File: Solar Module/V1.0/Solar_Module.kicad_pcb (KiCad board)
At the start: 4 copper layers, 23 parts, among them J1 B2B-PH-K-S, J2 TYPE-C16PIN, J3 B2B-PH-K-S, U1 MT3608, U2 TP4057

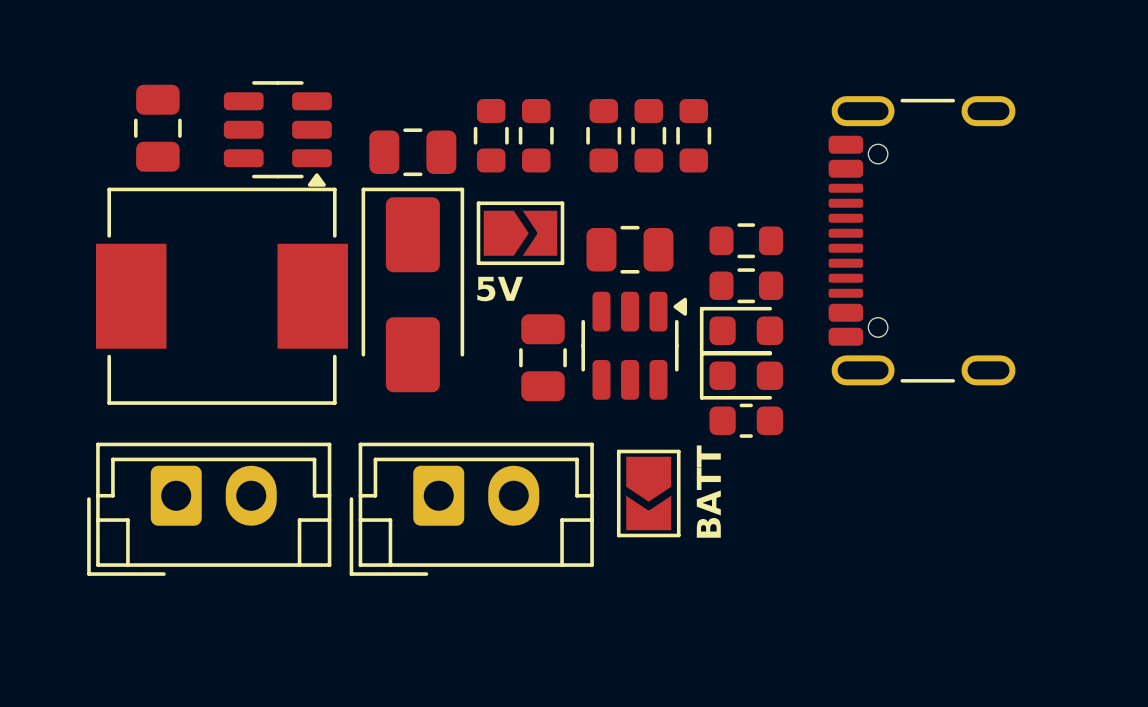
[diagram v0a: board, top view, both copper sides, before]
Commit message: Design roughly finished. Now Routing.
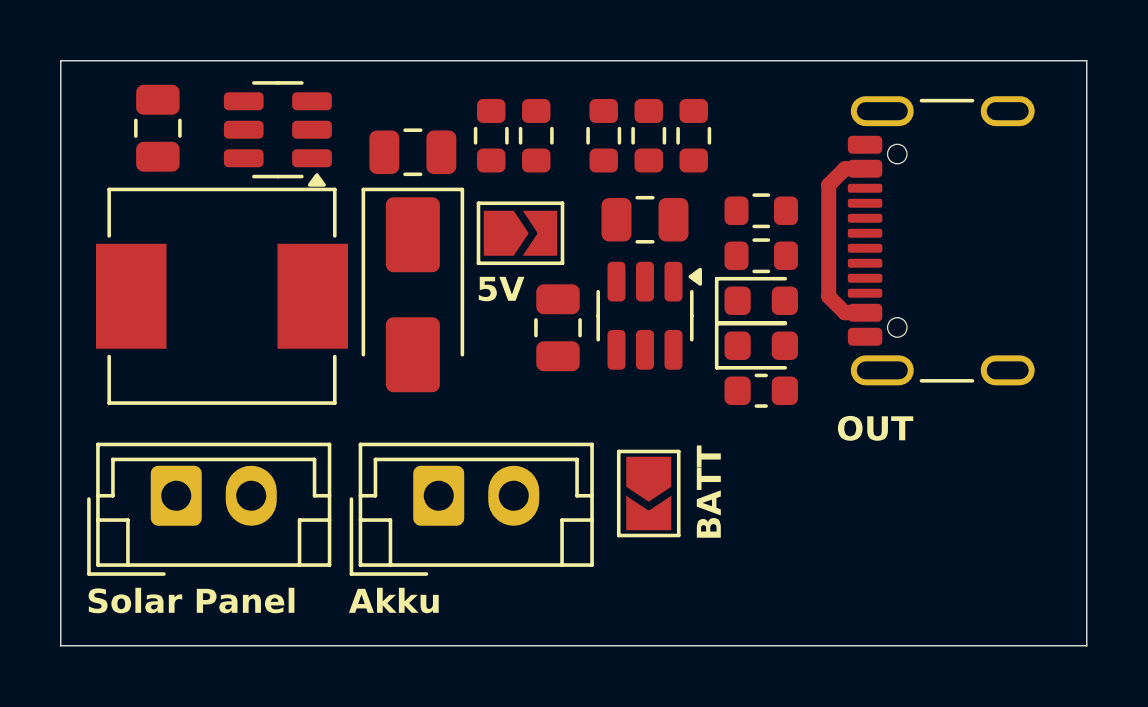
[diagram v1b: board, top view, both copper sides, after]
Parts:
- moved C3 1.12 mm to (168.0, 65.4)
- moved C4 1.12 mm to (170.9, 61.8)
- moved D2 1.12 mm to (174.8, 64.5)
- moved D3 1.12 mm to (174.8, 66.0)
- moved F1 1.12 mm to (174.8, 67.5)
- moved R3 1.12 mm to (174.8, 63.0)
- moved R4 1.12 mm to (174.8, 61.5)
- moved U2 1.12 mm to (170.9, 65.0)
- moved J2 0.64 mm to (181.9, 62.5)
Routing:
- net /VBUS_OUT: track 0.00 -> 6.59 mm
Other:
- board outline added: 34.2 x 19.5 mm
- board text added: "Akku"
- board text added: "OUT"
- board text added: "Solar Panel"
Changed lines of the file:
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@@
 	(footprint "LED_SMD:LED_0603_1608Metric"
 		(layer "F.Cu")
-		(at 174.250002 66.999999)
+		(at 174.750002 66)
 		(descr "LED SMD 0603 (1608 Metric), square (rectangular) end terminal, IPC_7351 nominal, (Body size source: http://www.tortai-tech.com/upload/download/2011102023233369053.pdf), generated with kicad-footprint-generator")
 		(tags "LED")
@@
 	(footprint "LED_SMD:LED_0603_1608Metric"
 		(layer "F.Cu")
-		(at 174.25 65.499999)
+		(at 174.75 64.5)
 		(descr "LED SMD 0603 (1608 Metric), square (rectangular) end terminal, IPC_7351 nominal, (Body size source: http://www.tortai-tech.com/upload/download/2011102023233369053.pdf), generated with kicad-footprint-generator")
 		(tags "LED")
@@
 	(footprint "Resistor_SMD:R_0603_1608Metric"
 		(layer "F.Cu")
-		(at 174.25 62.5)
+		(at 174.75 61.500001)
 		(descr "Resistor SMD 0603 (1608 Metric), square (rectangular) end terminal, IPC_7351 nominal, (Body size source: IPC-SM-782 page 72, https://www.pcb-3d.com/wordpress/wp-content/uploads/ipc-sm-782a_amendment_1_and_2.pdf), generated with kicad-footprint-generator")
 		(tags "resistor")
@@
 	(footprint "Capacitor_SMD:C_0805_2012Metric"
 		(layer "F.Cu")
-		(at 170.375002 62.799998)
+		(at 170.875002 61.799999)
 		(descr "Capacitor SMD 0805 (2012 Metric), square (rectangular) end terminal, IPC_7351 nominal, (Body size source: IPC-SM-782 page 76, https://www.pcb-3d.com/wordpress/wp-content/uploads/ipc-sm-782a_amendment_1_and_2.pdf, https://docs.google.com/spreadsheets/d/1BsfQQcO9C6DZCsRaXUlFlo91Tg2WpOkGARC1WS5S8t0/edit?usp=sharing), generated with kicad-footprint-generator")
 		(tags "capacitor")
@@
 	(footprint "Resistor_SMD:R_0603_1608Metric"
 		(layer "F.Cu")
-		(at 174.25 64)
+		(at 174.75 63.000001)
 		(descr "Resistor SMD 0603 (1608 Metric), square (rectangular) end terminal, IPC_7351 nominal, (Body size source: IPC-SM-782 page 72, https://www.pcb-3d.com/wordpress/wp-content/uploads/ipc-sm-782a_amendment_1_and_2.pdf), generated with kicad-footprint-generator")
 		(tags "resistor")
@@
 	(footprint "Package_TO_SOT_SMD:SOT-23-6"
 		(layer "F.Cu")
-		(at 170.375002 65.999998 -90)
+		(at 170.875002 64.999999 -90)
 		(descr "SOT, 6 Pin (https://www.jedec.org/sites/default/files/docs/Mo-178c.PDF variant AB), generated with kicad-footprint-generator ipc_gullwing_generator.py")
 		(tags "SOT TO_SOT_SMD")
@@
 	(footprint "Connector_USB:USB_C_Receptacle_GCT_USB4105-xx-A_16P_TopMnt_Horizontal"
 		(layer "F.Cu")
-		(at 181.25 62.5 90)
+		(at 181.89 62.5 90)
 		(descr "USB 2.0 Type C Receptacle, GCT, 16P, top mounted, horizontal, 5A: https://gct.co/files/drawings/usb4105.pdf")
 		(tags "USB C Type-C Receptacle SMD USB 2.0 16P 16C USB4105-15-A USB4105-15-A-060 USB4105-15-A-120 USB4105-GF-A USB4105-GF-A-060 USB4105-GF-A-120")
@@
 	(footprint "Fuse:Fuse_0603_1608Metric"
 		(layer "F.Cu")
-		(at 174.25 68.5)
+		(at 174.75 67.500001)
 		(descr "Fuse SMD 0603 (1608 Metric), square (rectangular) end terminal, IPC_7351 nominal, (Body size source: http://www.tortai-tech.com/upload/download/2011102023233369053.pdf), generated with kicad-footprint-generator")
 		(tags "fuse")
@@
 	(footprint "Capacitor_SMD:C_0805_2012Metric"
 		(layer "F.Cu")
-		(at 167.475002 66.399998 90)
+		(at 167.975002 65.399999 90)
 		(descr "Capacitor SMD 0805 (2012 Metric), square (rectangular) end terminal, IPC_7351 nominal, (Body size source: IPC-SM-782 page 76, https://www.pcb-3d.com/wordpress/wp-content/uploads/ipc-sm-782a_amendment_1_and_2.pdf, https://docs.google.com/spreadsheets/d/1BsfQQcO9C6DZCsRaXUlFlo91Tg2WpOkGARC1WS5S8t0/edit?usp=sharing), generated with kicad-footprint-generator")
 		(tags "capacitor")
@@
 		)
 	)
+	(gr_line
+		(start 185.6 76)
+		(end 185.6 56.5)
+		(stroke
+			(width 0.05)
+			(type default)
+		)
+		(layer "Edge.Cuts")
+	)
+	(gr_line
+		(start 151.4 56.5)
+		(end 151.4 76)
+		(stroke
+			(width 0.05)
+			(type default)
+		)
+		(layer "Edge.Cuts")
+	)
+	(gr_line
+		(start 151.4 76)
+		(end 185.6 76)
+		(stroke
+			(width 0.05)
+			(type default)
+		)
+		(layer "Edge.Cuts")
+	)
+	(gr_line
+		(start 185.6 56.5)
+		(end 151.4 56.5)
+		(stroke
+			(width 0.05)
+			(type default)
+		)
+		(layer "Edge.Cuts")
+	)
 	(gr_text "5V"
-		(at 165.2 64.6 0)
+		(at 165.25 64.6 0)
+		(layer "F.SilkS" knockout)
+		(effects
+			(font
+				(size 0.8 0.8)
+				(thickness 0.15)
+				(bold yes)
+			)
+			(justify left bottom)
+		)
+	)
+	(gr_text "Akku"
+		(at 161 75 0)
 		(layer "F.SilkS" knockout)
 		(effects
@@
 		)
 	)
+	(gr_text "Solar Panel"
+		(at 152.25 75 0)
+		(layer "F.SilkS" knockout)
+		(effects
+			(font
+				(size 0.8 0.8)
+				(thickness 0.15)
+				(bold yes)
+			)
+			(justify left bottom)
+		)
+	)
+	(gr_text "OUT"
+		(at 177.25 69.25 0)
+		(layer "F.SilkS" knockout)
+		(effects
+			(font
+				(size 0.8 0.8)
+				(thickness 0.15)
+				(bold yes)
+			)
+			(justify left bottom)
+		)
+	)
+	(segment
+		(start 178.21 60.1)
+		(end 177.540458 60.1)
+		(width 0.5)
+		(layer "F.Cu")
+		(net 14)
+	)
+	(segment
+		(start 177 64.359542)
+		(end 177.540458 64.9)
+		(width 0.5)
+		(layer "F.Cu")
+		(net 14)
+	)
+	(segment
+		(start 177.540458 60.1)
+		(end 177 60.640458)
+		(width 0.5)
+		(layer "F.Cu")
+		(net 14)
+	)
+	(segment
+		(start 177 60.640458)
+		(end 177 64.359542)
+		(width 0.5)
+		(layer "F.Cu")
+		(net 14)
+	)
+	(segment
+		(start 177.540458 64.9)
+		(end 178.21 64.9)
+		(width 0.5)
+		(layer "F.Cu")
+		(net 14)
+	)
 )
